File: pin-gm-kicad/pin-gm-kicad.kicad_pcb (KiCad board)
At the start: 2 copper layers, 62 x 45 mm, 40 parts, among them U1 LM358, U2 TL072

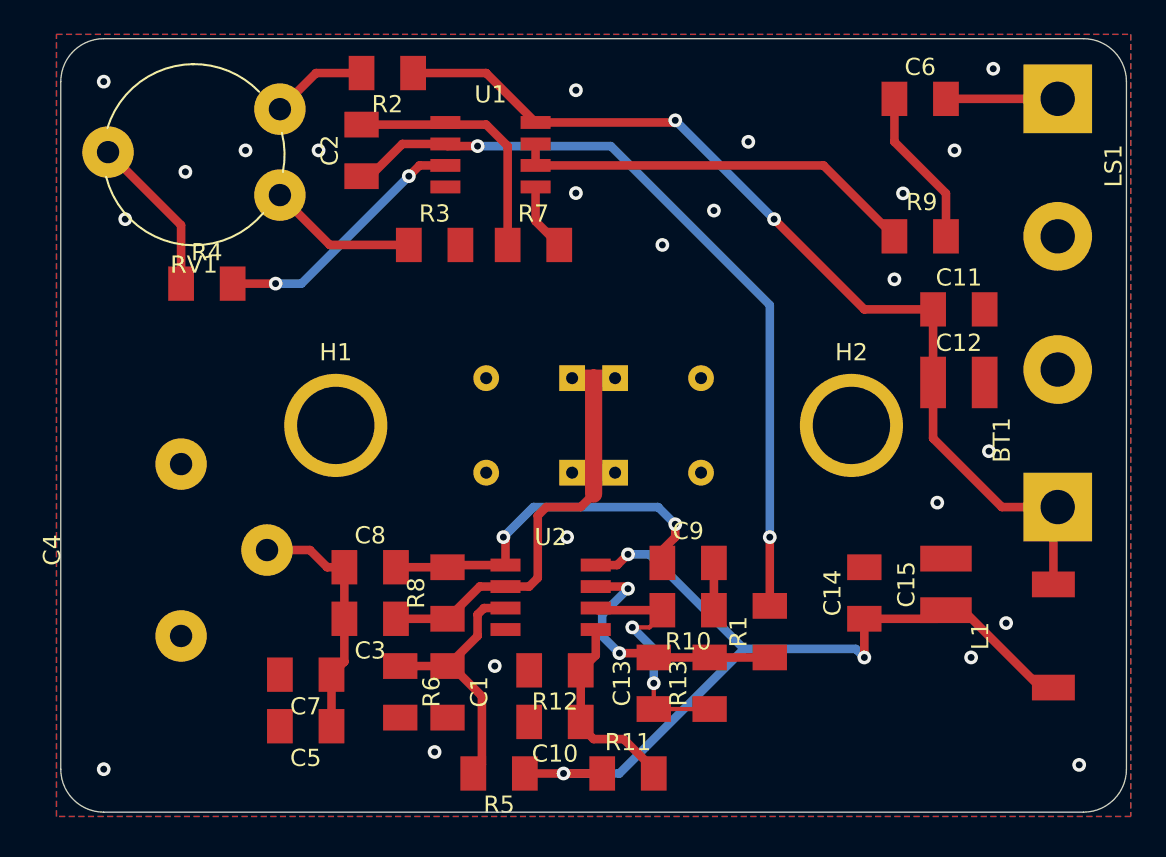
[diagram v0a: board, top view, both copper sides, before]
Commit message: mostmár tuti jó a layout
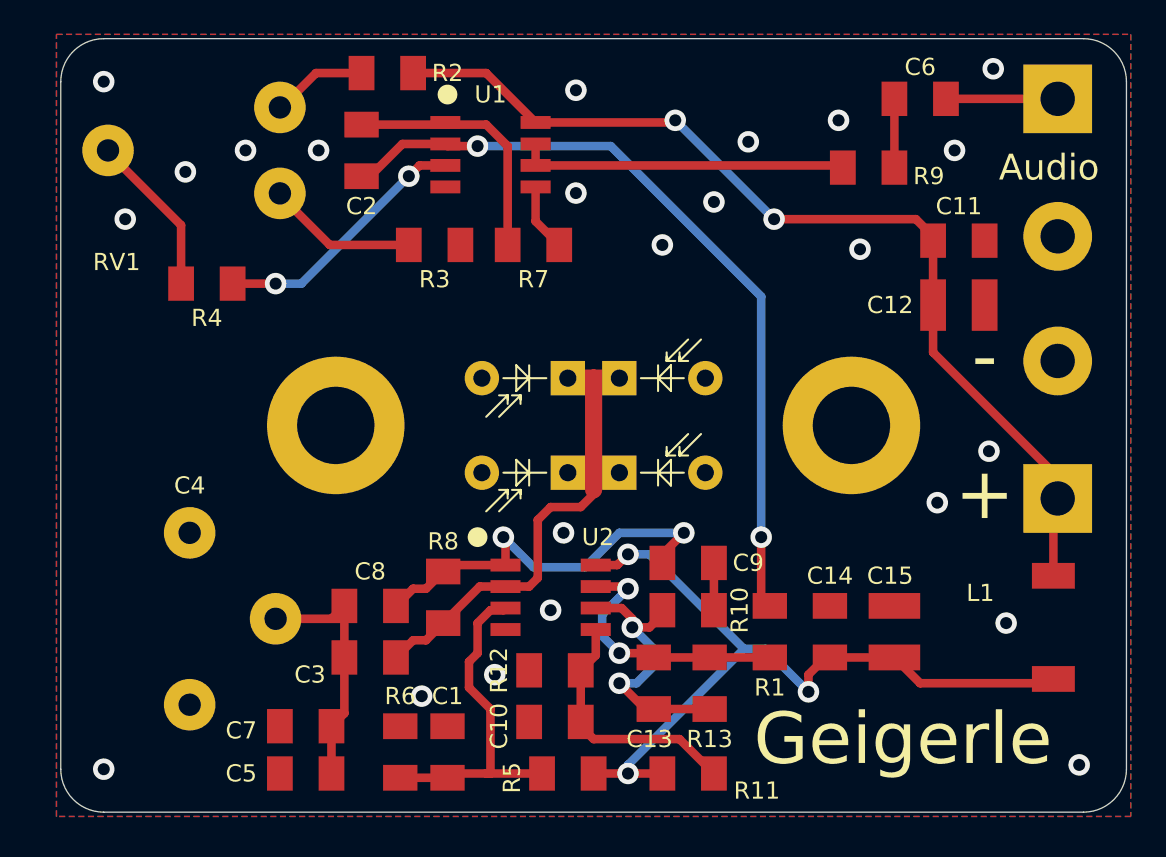
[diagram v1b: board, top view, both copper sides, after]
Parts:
- moved R9 5.00 mm to (101.0, 57.5)
- moved C12 4.50 mm to (106.2, 65.5)
- moved C15 4.07 mm to (102.5, 84.5)
- moved C4 4.03 mm to (61.5, 83.8)
- moved C11 4.00 mm to (106.2, 61.8)
- moved R5 4.00 mm to (83.5, 92.8)
- moved C1 3.50 mm to (76.5, 91.5), turned to 90 degrees
- moved R11 3.50 mm to (90.5, 92.8)
- moved R6 3.50 mm to (73.8, 91.5), turned to 90 degrees
- moved C14 3.01 mm to (98.8, 84.5)
- moved C7 3.00 mm to (68.2, 90.0)
- moved C5 2.75 mm to (68.2, 92.8)
- moved C3 2.25 mm to (72.0, 86.0)
- moved C8 2.25 mm to (72.0, 83.0)
- moved BT1 0.50 mm to (112.0, 76.8)
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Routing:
- net Net-(C14-Pad1): track 51.7 -> 46.4 mm
- net Net-(C6-Pad1): track 9.24 -> 4.00 mm
- net Net-(R9-Pad1): track 23.8 -> 19.2 mm
- net Net-(C1-Pad1): track 15.7 -> 19.8 mm
- net Net-(C10-Pad1): track 11.5 -> 14.9 mm
- net Net-(C13-Pad1): track 14.8 -> 16.2 mm
- net /Diode_Cathode: track 28.4 -> 29.8 mm
- net Net-(C8-Pad2): track 21.8 -> 23.0 mm
- net VCC: track 57.6 -> 56.8 mm
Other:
- board text added: "+"
- board text added: "-"
- board text added: "Audio"
- board text added: "Geigerle"
